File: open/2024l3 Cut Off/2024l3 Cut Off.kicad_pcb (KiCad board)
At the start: 2 copper layers, 140 x 100 mm, 24 parts, among them J1 Conn_01x06, J2 TOF 0, J3 TOF 1, J4 TOF 2, J5 TOF 3, U1 OpenMV, U2 4754, U3 xiao-esp32c3, U4 Adafruit Featherwing, U5 Teensy 4.0

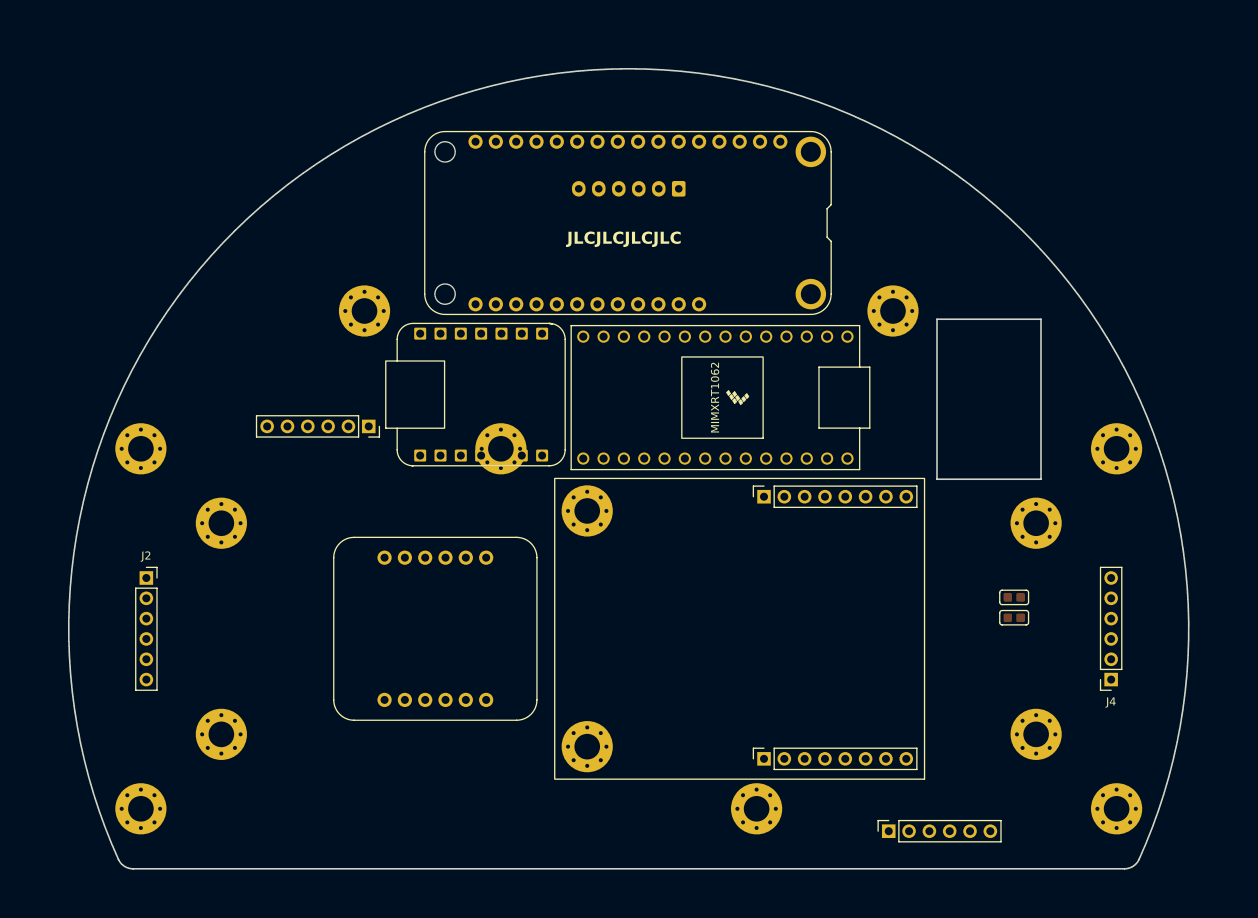
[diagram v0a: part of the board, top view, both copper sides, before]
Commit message: L3 Temp Placement
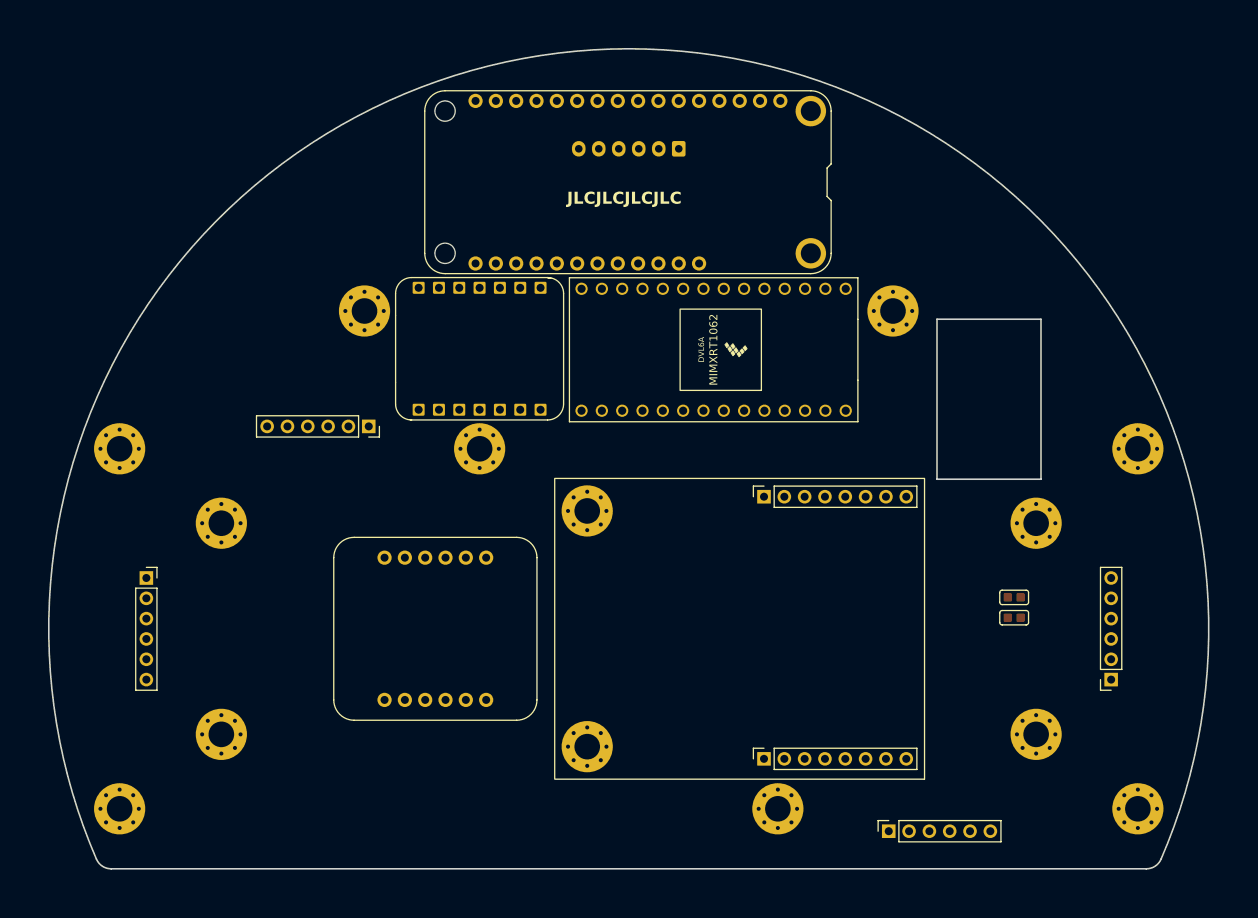
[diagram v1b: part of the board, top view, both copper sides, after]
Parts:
- U3: value xiao-esp32c3 -> >VALUE
- moved Ue 5.98 mm to (159.1, 70.1)
- moved U3 5.73 mm to (129.9, 70.0)
- moved U4 5.10 mm to (148.5, 49.1)
- moved J1 5.00 mm to (154.7, 45.0)
- moved H3 2.66 mm to (84.9, 127.5)
- moved H12 2.66 mm to (84.9, 82.5)
- moved H9 2.66 mm to (212.1, 82.5)
- moved H11 2.66 mm to (212.1, 127.5)
- moved H4 2.66 mm to (167.1, 127.5)
- moved H10 2.66 mm to (129.9, 82.5)
- renumbered U5 to Ue
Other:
- board size 140 x 100 mm -> 145 x 102.5 mm
